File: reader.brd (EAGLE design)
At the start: 49.5 x 35.6 mm, 16 parts, among them J1 RJ11-6PTH, J2 AVR_SPI_PRG_6NS, T1 BC547

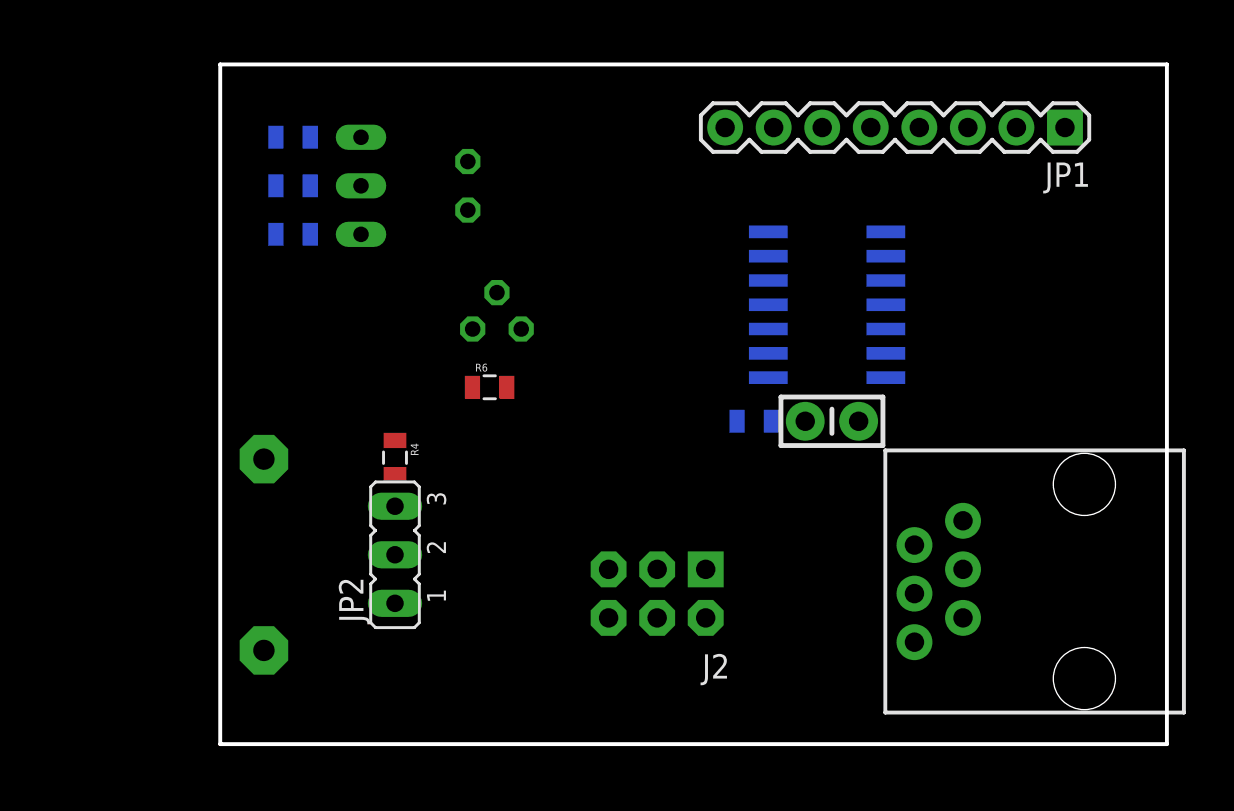
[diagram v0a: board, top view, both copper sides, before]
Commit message: [WIP] Manually route few connectors on the board
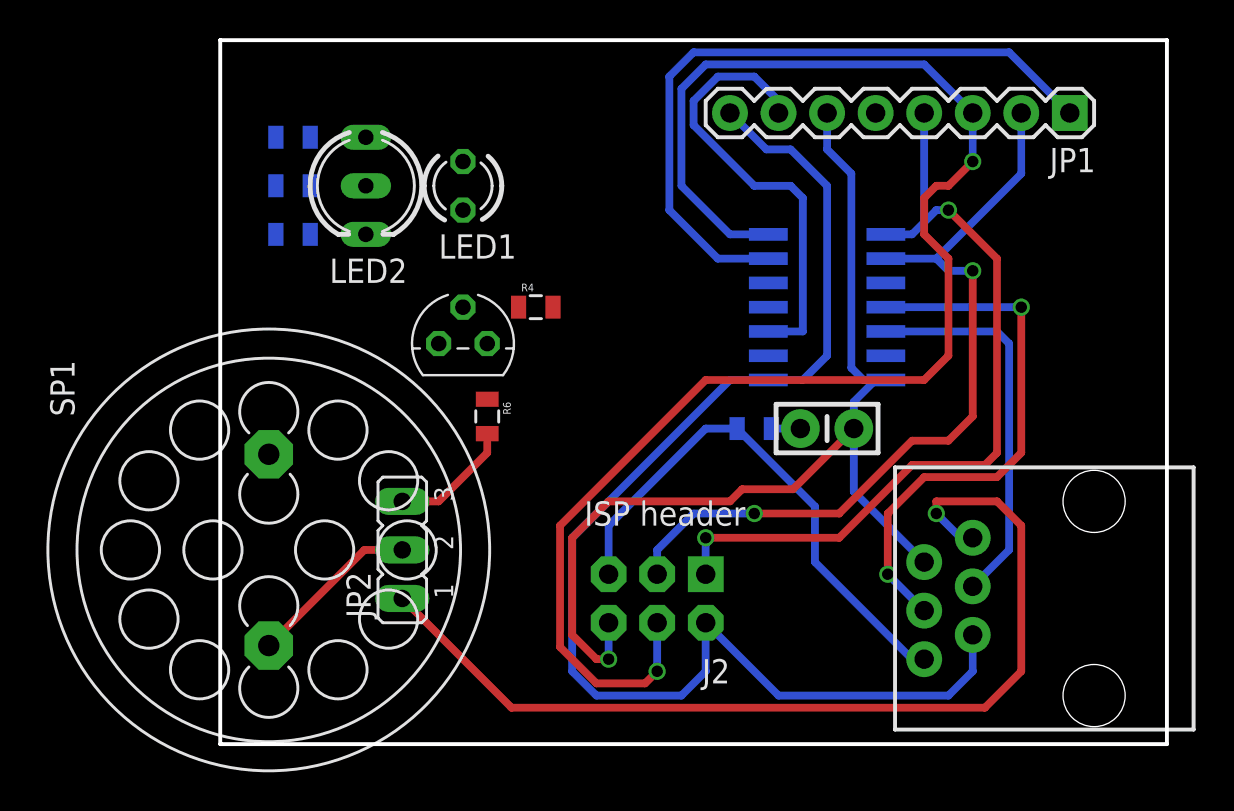
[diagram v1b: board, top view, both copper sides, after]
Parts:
- removed LD1: STATUS, led:DUOLED-C-5MM
- removed U$1: TINY841, attiny841:SO14
- added LED2: STATUS, led:DUOLED-C-5MM
- added U1: TINY841, attiny841:SO14
- moved R4 10.8 mm to (16.5, 22.9), turned to 0 degrees
- moved T1 1.93 mm to (12.7, 21.0), flipped to the top
- moved R6 1.53 mm to (14.0, 17.1), turned to 270 degrees
- moved J1 1.02 mm to (45.7, 2.54)
- moved JP1 0.80 mm to (44.5, 33.0)
- moved JP2 0.46 mm to (9.53, 10.2)
- moved C1 0.46 mm to (31.8, 16.5)
- moved R5 0.38 mm to (27.9, 16.5)
- moved SP1 0.36 mm to (2.54, 10.2), flipped to the top
- moved LED1 0.25 mm to (12.7, 29.2), flipped to the top
- moved J2 0.25 mm to (22.9, 7.62)
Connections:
- net BLUE_LED: now also U1.13; no longer U$1.13
- net CONTROLLER_RXD: now also U1.11; no longer U$1.11
- net CONTROLLER_TXD: now also U1.12; no longer U$1.12
- net GND: now also LED2.C, U1.14; no longer LD1.C, U$1.14
- net GREEN_LED: now also U1.5; no longer U$1.5
- net MISO: now also U1.8; no longer U$1.8
- net MOSI: now also U1.7; no longer U$1.7
- net N$2: now also LED2.AR; no longer LD1.AR
- net N$3: now also LED2.AX; no longer LD1.AX
- net RDR_RESET: now also U1.3; no longer U$1.3
- net RDR_SS: now also U1.6; no longer U$1.6
- net RED_LED: now also U1.2; no longer U$1.2
- net RST: now also U1.4; no longer U$1.4
- net SCK: now also U1.9; no longer U$1.9
- net SPEAKER: now also U1.10; no longer U$1.10
- net VCC: now also U1.1; no longer U$1.1
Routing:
- net MOSI: track 0.00 -> 81.2 mm, vias 0 -> 2
- net VCC: track 0.00 -> 69.9 mm
- net GND: track 0.00 -> 54.5 mm, vias 0 -> 1
- net EXT_SPEAKER: track 0.00 -> 51.2 mm, vias 0 -> 1
- net SCK: track 0.00 -> 42.6 mm, vias 0 -> 2
- net MISO: track 0.00 -> 42.3 mm, vias 0 -> 2
- net RDR_SS: track 0.00 -> 36.0 mm
- net CONTROLLER_RXD: track 0.00 -> 28.9 mm, vias 0 -> 2
- net RST: track 0.00 -> 27.9 mm
- net RDR_RESET: track 0.00 -> 23.5 mm
- net CONTROLLER_TXD: track 0.00 -> 20.2 mm
- net N$1: track 0.00 -> 9.06 mm
- net N$7: track 0.00 -> 6.50 mm
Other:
- board size 49.5 x 35.6 mm -> 49.5 x 36.8 mm
- board text added: "* *-* internal *-* * external"
- board text added: "ISP header"
- board text added: "LED2"
- board text added: "Read"
- board text added: "Status"
